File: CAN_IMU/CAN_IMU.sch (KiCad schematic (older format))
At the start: 12 parts

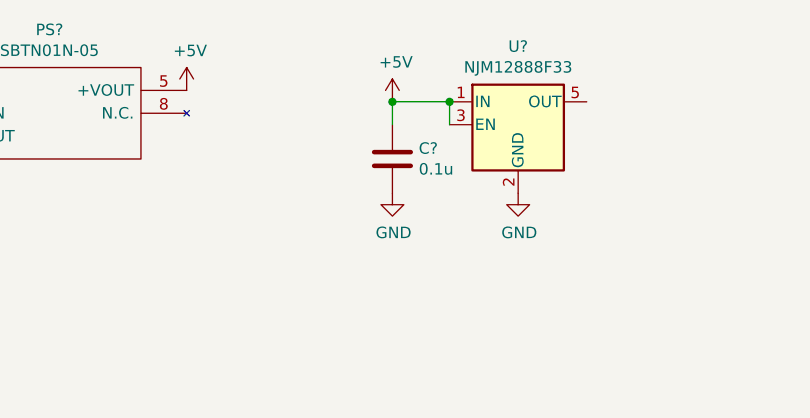
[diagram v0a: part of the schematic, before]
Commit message: move
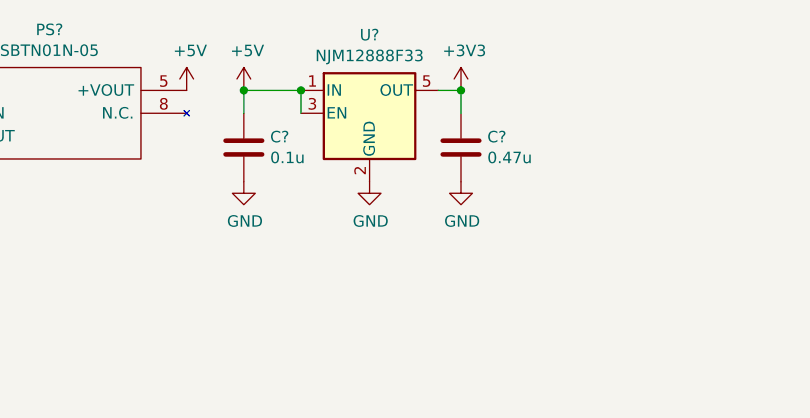
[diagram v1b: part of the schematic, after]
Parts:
- added C?: 0.47u, Capacitor_SMD:C_0603_1608Metric_Pad1.05x0.95mm_HandSolder, symbol Device:C
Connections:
- net +3V3: now also U?.5 (OUT), C?.1
- net GND: now also C?.2
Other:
- moved on the sheet: C?, U?
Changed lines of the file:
@@
 L Regulator_Linear:TLV70212_SOT23-5 U?
 U 1 1 5DE7821C
-P 3900 1050
-F 0 "U?" H 3900 1392 50  0000 C CNN
-F 1 "NJM12888F33" H 3900 1301 50  0000 C CNN
-F 2 "Package_TO_SOT_SMD:SOT-23-5" H 3900 1375 50  0001 C CIN
-F 3 "http://www.ti.com/lit/ds/symlink/tlv702.pdf" H 3900 1100 50  0001 C CNN
-	1    3900 1050
+P 3250 1000
+F 0 "U?" H 3250 1342 50  0000 C CNN
+F 1 "NJM12888F33" H 3250 1251 50  0000 C CNN
+F 2 "Package_TO_SOT_SMD:SOT-23-5" H 3250 1325 50  0001 C CIN
+F 3 "http://www.ti.com/lit/ds/symlink/tlv702.pdf" H 3250 1050 50  0001 C CNN
+	1    3250 1000
 	1    0    0    -1
 $EndComp
@@
 L Device:C C?
 U 1 1 5DE78FD8
-P 3350 1200
-F 0 "C?" H 3465 1246 50  0000 L CNN
-F 1 "0.1u" H 3465 1155 50  0000 L CNN
-F 2 "Capacitor_SMD:C_0603_1608Metric_Pad1.05x0.95mm_HandSolder" H 3388 1050 50  0001 C CNN
-F 3 "~" H 3350 1200 50  0001 C CNN
-	1    3350 1200
+P 2700 1150
+F 0 "C?" H 2815 1196 50  0000 L CNN
+F 1 "0.1u" H 2815 1105 50  0000 L CNN
+F 2 "Capacitor_SMD:C_0603_1608Metric_Pad1.05x0.95mm_HandSolder" H 2738 1000 50  0001 C CNN
+F 3 "~" H 2700 1150 50  0001 C CNN
+	1    2700 1150
 	1    0    0    -1
 $EndComp
 Wire Wire Line
-	3600 1050 3600 950
+	2950 1000 2950 900
 $Comp
 L power:+5V #PWR?
 U 1 1 5DE7AC64
-P 3350 950
-F 0 "#PWR?" H 3350 800 50  0001 C CNN
-F 1 "+5V" H 3365 1123 50  0000 C CNN
-F 2 "" H 3350 950 50  0001 C CNN
-F 3 "" H 3350 950 50  0001 C CNN
-	1    3350 950
+P 2700 900
+F 0 "#PWR?" H 2700 750 50  0001 C CNN
+F 1 "+5V" H 2715 1073 50  0000 C CNN
+F 2 "" H 2700 900 50  0001 C CNN
+F 3 "" H 2700 900 50  0001 C CNN
+	1    2700 900
 	1    0    0    -1
 $EndComp
@@
 L power:GND #PWR?
 U 1 1 5DE7B2E4
-P 3350 1350
-F 0 "#PWR?" H 3350 1100 50  0001 C CNN
-F 1 "GND" H 3355 1177 50  0000 C CNN
-F 2 "" H 3350 1350 50  0001 C CNN
-F 3 "" H 3350 1350 50  0001 C CNN
-	1    3350 1350
+P 2700 1300
+F 0 "#PWR?" H 2700 1050 50  0001 C CNN
+F 1 "GND" H 2705 1127 50  0000 C CNN
+F 2 "" H 2700 1300 50  0001 C CNN
+F 3 "" H 2700 1300 50  0001 C CNN
+	1    2700 1300
 	1    0    0    -1
 $EndComp
@@
 L power:GND #PWR?
 U 1 1 5DE7B63B
-P 3900 1350
-F 0 "#PWR?" H 3900 1100 50  0001 C CNN
-F 1 "GND" H 3905 1177 50  0000 C CNN
-F 2 "" H 3900 1350 50  0001 C CNN
-F 3 "" H 3900 1350 50  0001 C CNN
-	1    3900 1350
+P 3250 1300
+F 0 "#PWR?" H 3250 1050 50  0001 C CNN
+F 1 "GND" H 3255 1127 50  0000 C CNN
+F 2 "" H 3250 1300 50  0001 C CNN
+F 3 "" H 3250 1300 50  0001 C CNN
+	1    3250 1300
 	1    0    0    -1
 $EndComp
 Wire Wire Line
-	3600 950  3350 950
+	2950 900  2700 900
 Wire Wire Line
-	3350 950  3350 1050
-Connection ~ 3600 950
-Connection ~ 3350 950
+	2700 900  2700 1000
+Connection ~ 2950 900
+Connection ~ 2700 900
+$Comp
+L power:+3V3 #PWR?
+U 1 1 5DE7C8AB
+P 3650 900
+F 0 "#PWR?" H 3650 750 50  0001 C CNN
+F 1 "+3V3" H 3665 1073 50  0000 C CNN
+F 2 "" H 3650 900 50  0001 C CNN
+F 3 "" H 3650 900 50  0001 C CNN
+	1    3650 900
+	1    0    0    -1
+$EndComp
+$Comp
+L Device:C C?
+U 1 1 5DE7D144
+P 3650 1150
+F 0 "C?" H 3765 1196 50  0000 L CNN
+F 1 "0.47u" H 3765 1105 50  0000 L CNN
+F 2 "Capacitor_SMD:C_0603_1608Metric_Pad1.05x0.95mm_HandSolder" H 3688 1000 50  0001 C CNN
+F 3 "~" H 3650 1150 50  0001 C CNN
+	1    3650 1150
+	1    0    0    -1
+$EndComp
+Wire Wire Line
+	3650 1000 3650 900
+Wire Wire Line
+	3650 900  3550 900
+Connection ~ 3650 900
+$Comp
+L power:GND #PWR?
+U 1 1 5DE7E724
+P 3650 1300
+F 0 "#PWR?" H 3650 1050 50  0001 C CNN
+F 1 "GND" H 3655 1127 50  0000 C CNN
+F 2 "" H 3650 1300 50  0001 C CNN
+F 3 "" H 3650 1300 50  0001 C CNN
+	1    3650 1300
+	1    0    0    -1
+$EndComp
 $EndSCHEMATC

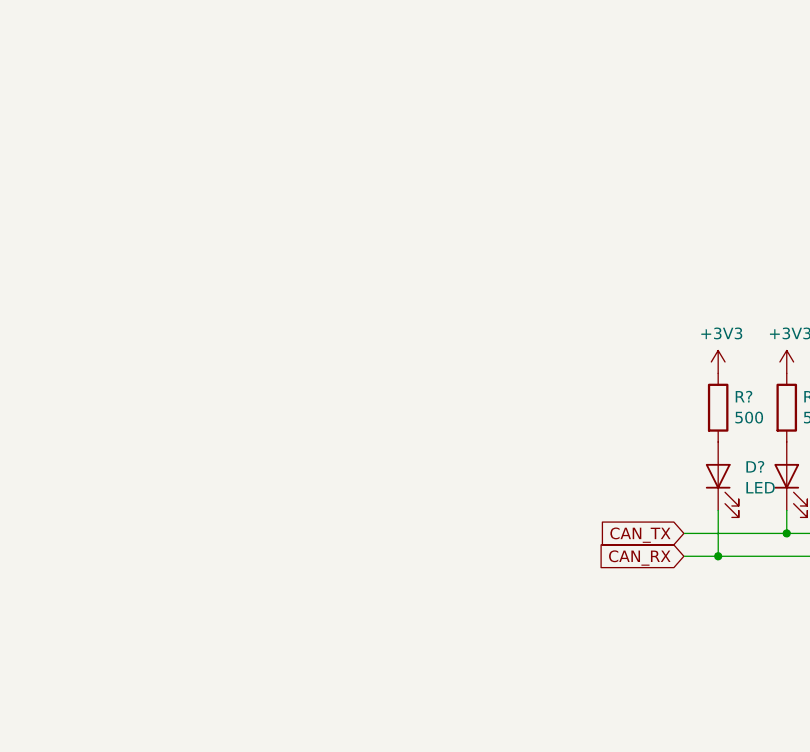
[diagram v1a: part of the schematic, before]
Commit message: micon
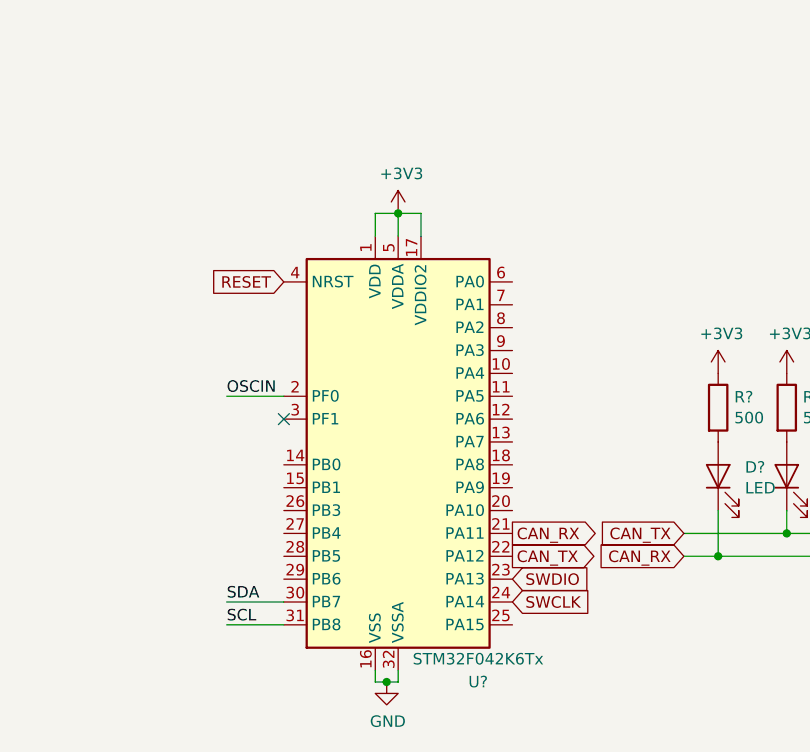
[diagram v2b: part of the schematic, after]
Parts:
- added U?: STM32F042K6Tx, Package_QFP:LQFP-32_7x7mm_P0.8mm, symbol MCU_ST_STM32F0:STM32F042K6Tx
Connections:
- net +3V3: now also U?.1 (VDD), U?.17 (VDDIO2), U?.5 (VDDA)
- net CAN_RX: now also U?.21 (PA11)
- net CAN_TX: now also U?.22 (PA12)
- net GND: now also U?.16 (VSS), U?.32 (VSSA)
- new net OSCIN: U?.2 (PF0)
- new net RESET: U?.4 (NRST)
- new net SCL: U?.31 (PB8)
- new net SDA: U?.30 (PB7)
- new net SWCLK: U?.24 (PA14)
- new net SWDIO: U?.23 (PA13)
- no-connect marks 0 -> 1
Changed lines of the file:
@@
 	1    0    0    -1
 $EndComp
+$Comp
+L MCU_ST_STM32F0:STM32F042K6Tx U?
+U 1 1 5DE77FCA
+P 3200 3800
+F 0 "U?" H 3550 2750 50  0000 C CNN
+F 1 "STM32F042K6Tx" H 3550 2850 50  0000 C CNN
+F 2 "Package_QFP:LQFP-32_7x7mm_P0.8mm" H 2800 2900 50  0001 R CNN
+F 3 "http://www.st.com/st-web-ui/static/active/en/resource/technical/document/datasheet/DM00105814.pdf" H 3200 3800 50  0001 C CNN
+	1    3200 3800
+	1    0    0    -1
+$EndComp
+$Comp
+L power:+3V3 #PWR?
+U 1 1 5DE7A1A5
+P 3200 2800
+F 0 "#PWR?" H 3200 2650 50  0001 C CNN
+F 1 "+3V3" H 3215 2973 50  0000 C CNN
+F 2 "" H 3200 2800 50  0001 C CNN
+F 3 "" H 3200 2800 50  0001 C CNN
+	1    3200 2800
+	1    0    0    -1
+$EndComp
+Wire Wire Line
+	3300 2900 3300 2800
+Wire Wire Line
+	3300 2800 3200 2800
+Wire Wire Line
+	3100 2800 3100 2900
+Connection ~ 3200 2800
+Wire Wire Line
+	3200 2800 3100 2800
+Wire Wire Line
+	3200 2900 3200 2800
+$Comp
+L power:GND #PWR?
+U 1 1 5DE7B378
+P 3150 4850
+F 0 "#PWR?" H 3150 4600 50  0001 C CNN
+F 1 "GND" H 3155 4677 50  0000 C CNN
+F 2 "" H 3150 4850 50  0001 C CNN
+F 3 "" H 3150 4850 50  0001 C CNN
+	1    3150 4850
+	1    0    0    -1
+$EndComp
+Wire Wire Line
+	3200 4800 3200 4850
+Wire Wire Line
+	3200 4850 3150 4850
+Wire Wire Line
+	3100 4800 3100 4850
+Wire Wire Line
+	3100 4850 3150 4850
+Connection ~ 3150 4850
+Text Label 2450 3600 0    50   ~ 0
+OSCIN
+Wire Wire Line
+	2450 3600 2700 3600
+NoConn ~ 2700 3700
+Text Label 2450 4600 0    50   ~ 0
+SCL
+Text Label 2450 4500 0    50   ~ 0
+SDA
+Wire Wire Line
+	2450 4500 2700 4500
+Wire Wire Line
+	2700 4600 2450 4600
+Text GLabel 3700 4300 2    50   Output ~ 0
+CAN_TX
+Text GLabel 3700 4200 2    50   Output ~ 0
+CAN_RX
+Text GLabel 3700 4400 2    50   Input ~ 0
+SWDIO
+Text GLabel 3700 4500 2    50   Input ~ 0
+SWCLK
+Text GLabel 2700 3100 0    50   Input ~ 0
+RESET
 $EndSCHEMATC
